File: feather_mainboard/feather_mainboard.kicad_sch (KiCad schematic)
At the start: 0 parts

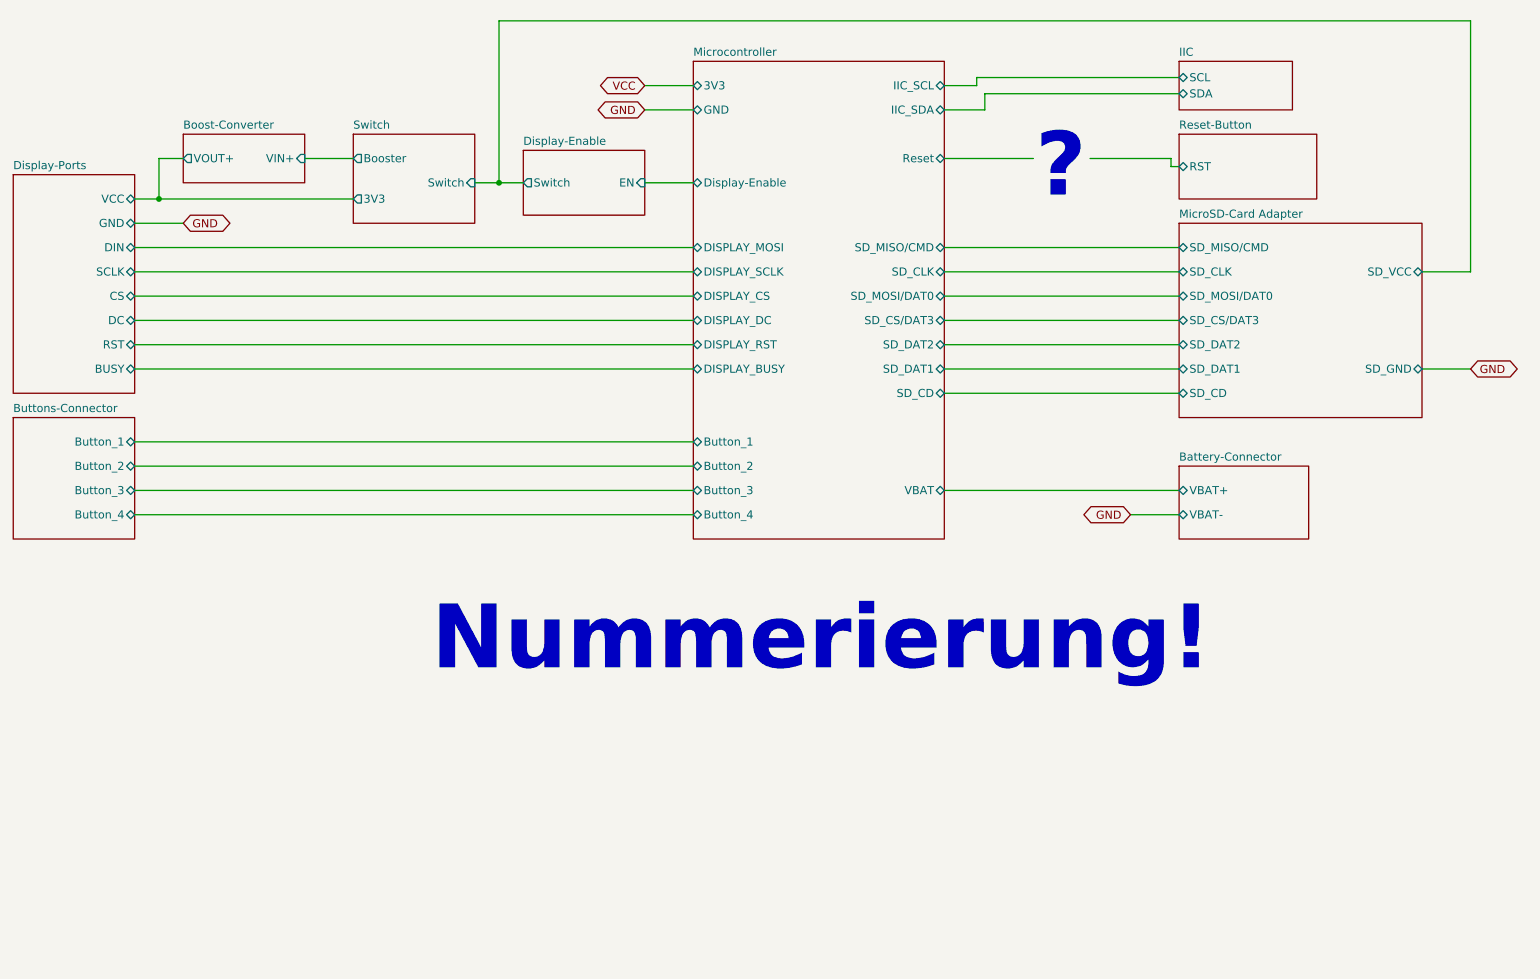
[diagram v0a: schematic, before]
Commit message: finished mainboard design, need to do the routing
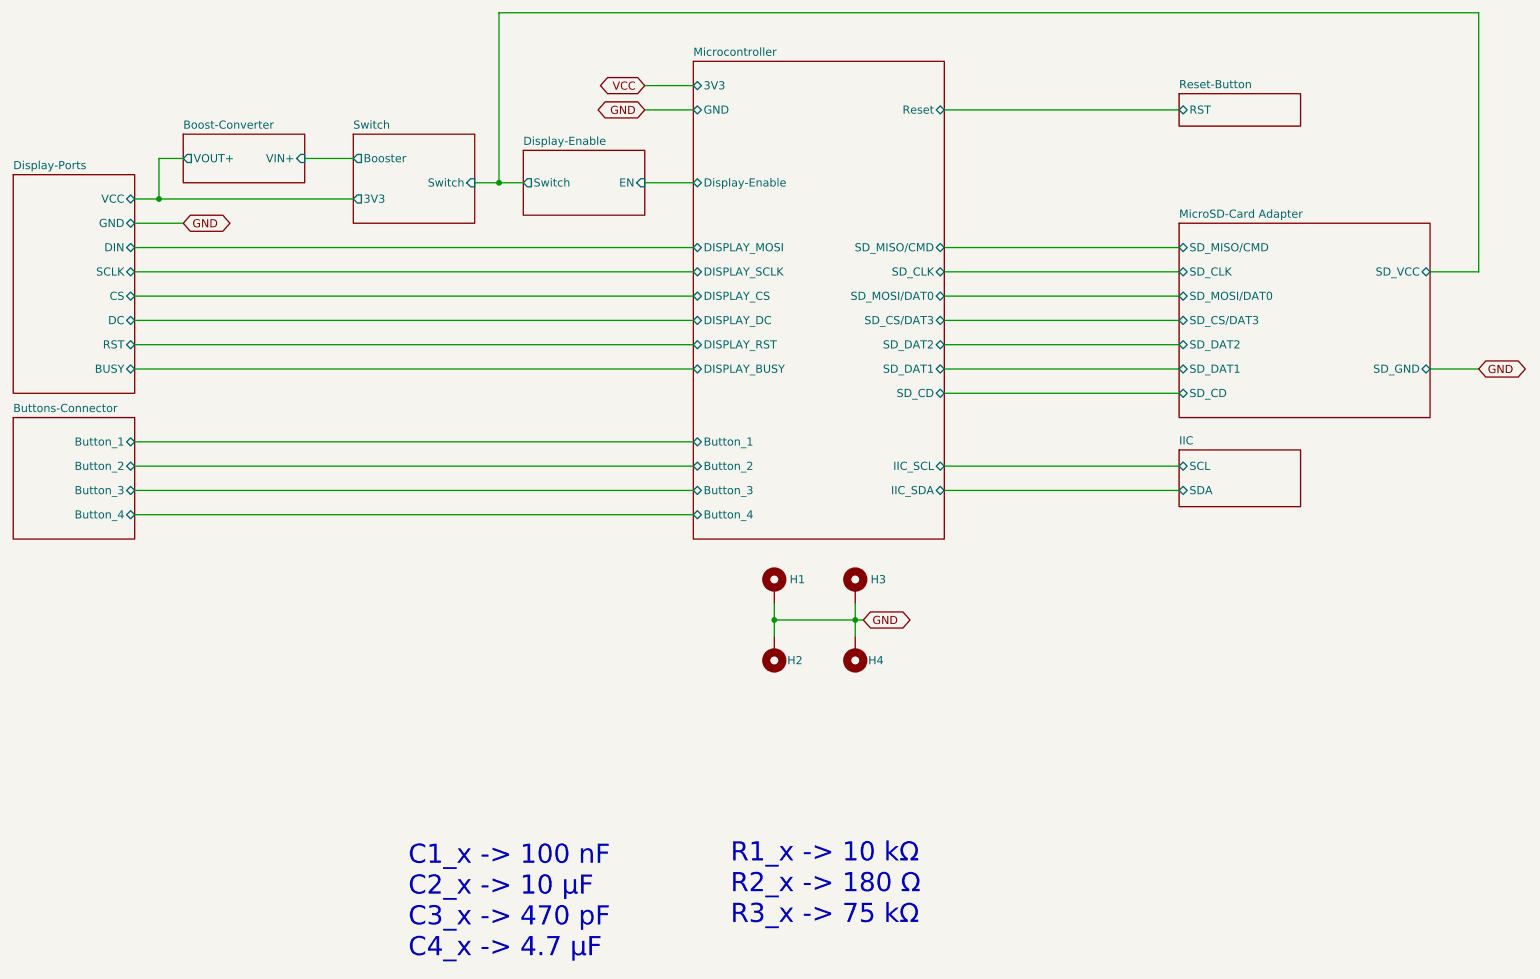
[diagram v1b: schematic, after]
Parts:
- added H1, H2, H3, H4: MountingHole_Pad, MountingHole:MountingHole_2.2mm_M2_DIN965_Pad, symbol Mechanical:MountingHole_Pad
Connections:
- net GND: now also H1.1, H2.1, H3.1, H4.1
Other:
- removed sheet Battery-Connector
- sheet Microcontroller ports: added none; removed VBAT
- note added: "C1_x -> 100 nF C2_x -> 10 µF C3_x -> 470 pF C4_x -> 4.7 µF"
- note added: "R1_x -> 10 kΩ R2_x -> 180 Ω R3_x -> 75 kΩ"
- note removed: "?"
- note removed: "Nummerierung!"
